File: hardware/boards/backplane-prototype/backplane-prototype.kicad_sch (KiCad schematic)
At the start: 32 parts, among them J1 SLOT_1, J2 i2c_busses, J3 SLOT_2, J4 SLOT_3, J5 DC_IN, J6 SLOT_4, J7 SLOT_5, J8 SLOT_6

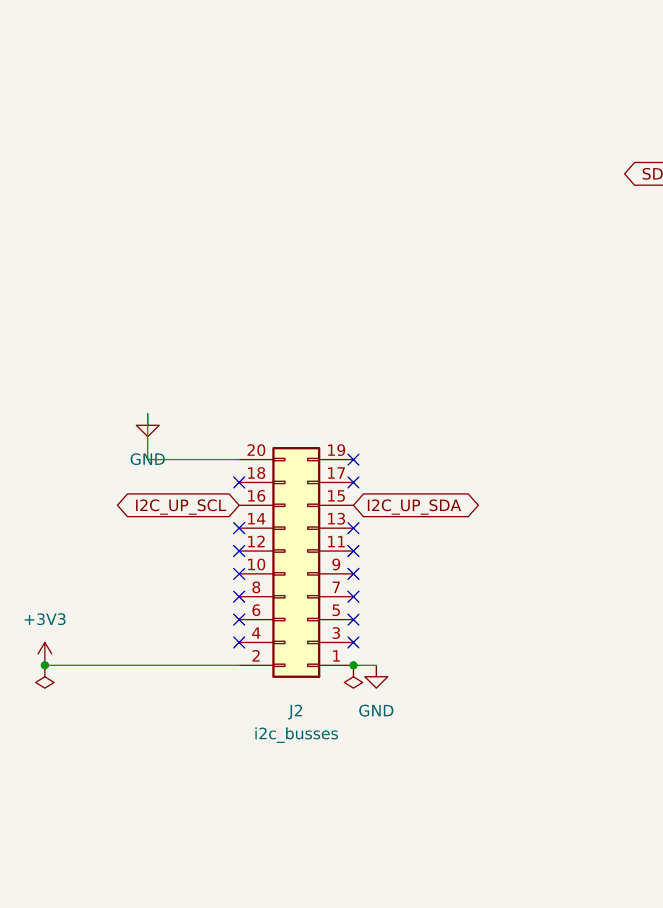
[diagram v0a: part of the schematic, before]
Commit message: Checkpoint before auto-router
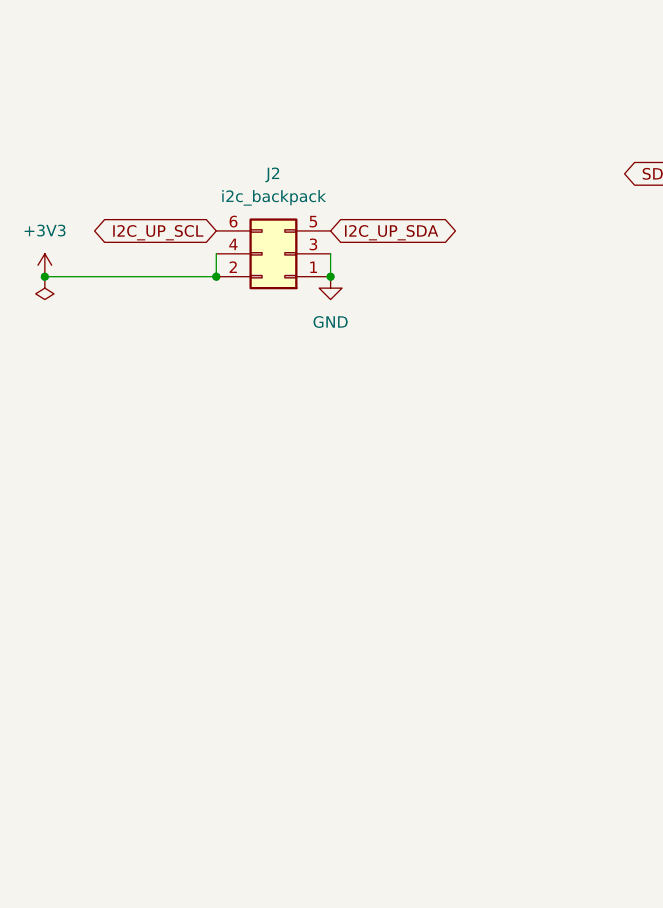
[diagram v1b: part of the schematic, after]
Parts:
- J2: value i2c_busses -> i2c_backpack; footprint Connector_PinHeader_1.00mm:PinHeader_2x10_P1.00mm_Vertical -> Connector_PinHeader_2.54mm:PinHeader_2x03_P2.54mm_Vertical; symbol Connector_Generic:Conn_02x10_Odd_Even -> Connector_Generic:Conn_02x03_Odd_Even
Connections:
- net +3V3: now also J2.4 (Pin_4)
- net GND: now also J2.3 (Pin_3); no longer J2.20 (Pin_20)
- net I2C_UP_SCL: now also J2.6 (Pin_6); no longer J2.16 (Pin_16)
- net I2C_UP_SDA: now also J2.5 (Pin_5); no longer J2.15 (Pin_15)
- no-connect marks 15 -> 0
